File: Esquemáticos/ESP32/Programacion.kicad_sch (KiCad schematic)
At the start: 10 parts, among them U7 ESP32-WROOM-32

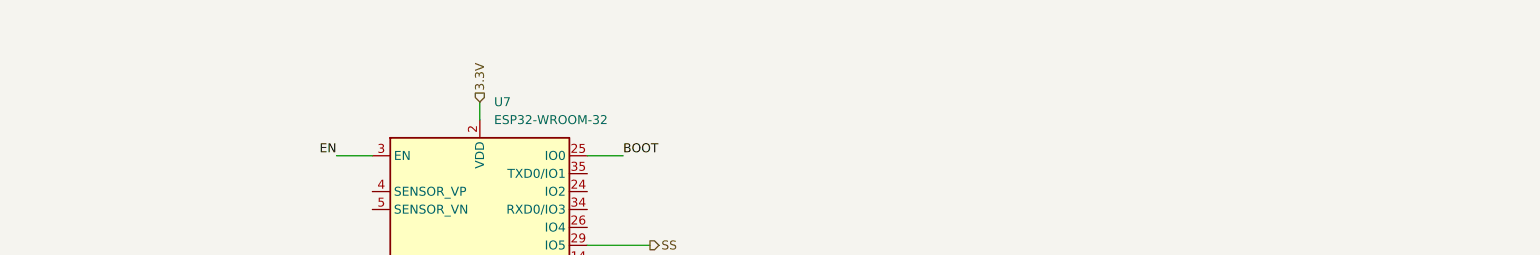
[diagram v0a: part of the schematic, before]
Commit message: Push mid :V
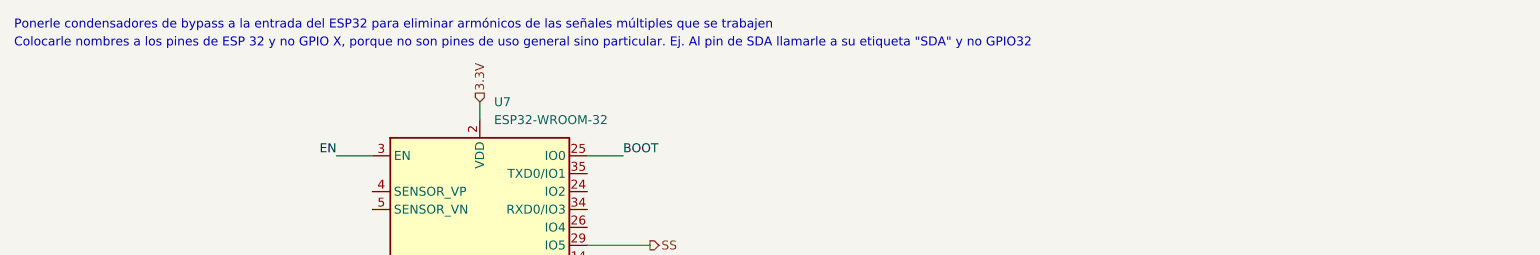
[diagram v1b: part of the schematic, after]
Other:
- note added: "Colocarle nombres a los pines de ESP 32 y no GPIO X, porque no son pines de uso general sino particular. Ej. Al pin de SDA llamarle a su etiqueta "SDA" y no GPIO32"
- note added: "Ponerle condensadores de bypass a la entrada del ESP32 para eliminar armónicos de las señales múltiples que se trabajen"
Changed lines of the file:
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@@
+    (effects (font (size 1.27 1.27)) (justify left bottom))
+  )
+  (text "Ponerle condensadores de bypass a la entrada del ESP32 para eliminar armónicos de las señales múltiples que se trabajen\n"
+    (at 29.21 44.45 0)
+    (effects (font (size 1.27 1.27)) (justify left bottom))
+  )
+  (text "Colocarle nombres a los pines de ESP 32 y no GPIO X, porque no son pines de uso general sino particular. Ej. Al pin de SDA llamarle a su etiqueta \"SDA\" y no GPIO32"
+    (at 29.21 46.99 0)
     (effects (font (size 1.27 1.27)) (justify left bottom))
   )
